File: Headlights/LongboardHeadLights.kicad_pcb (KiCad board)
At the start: 2 copper layers, 76.2 x 12.7 mm, 16 parts, among them P1 CONN_01X03, U1 AL8805

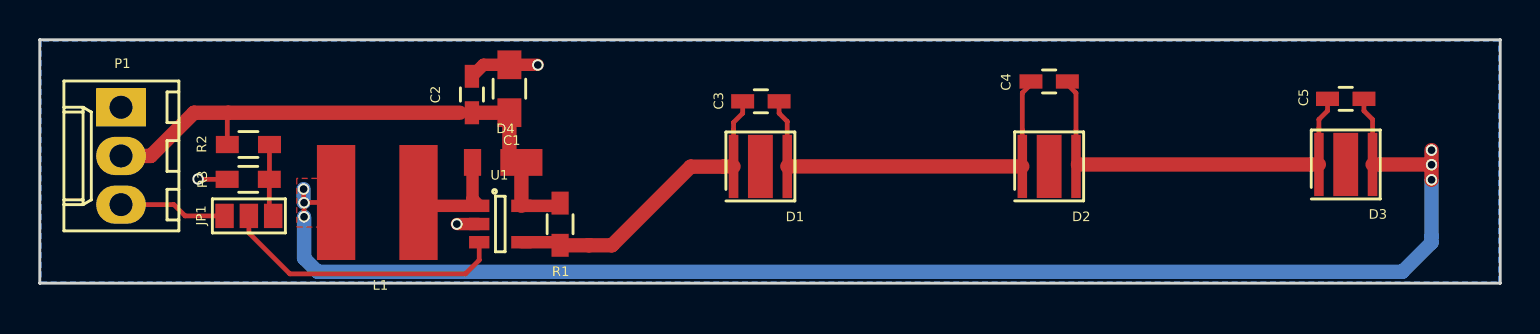
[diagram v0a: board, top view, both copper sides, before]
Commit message: updated project and completed rev 1 PCB
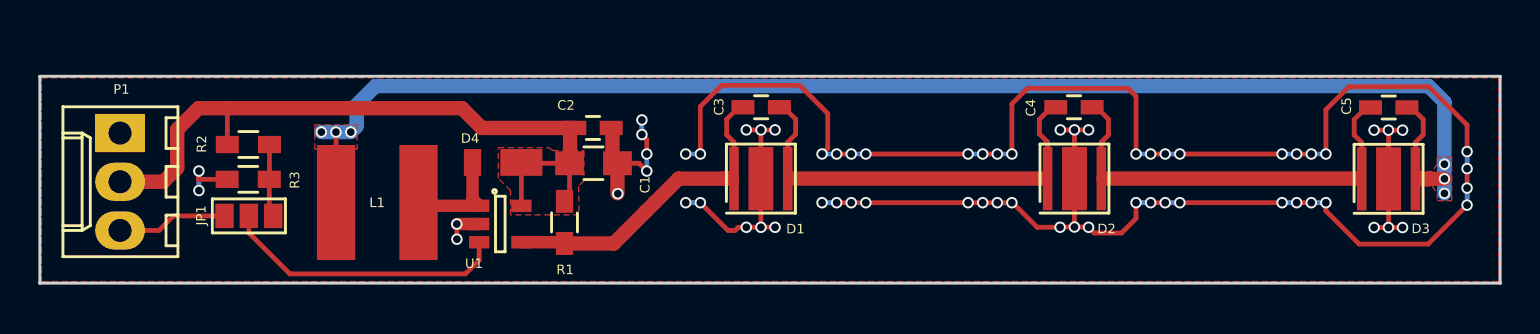
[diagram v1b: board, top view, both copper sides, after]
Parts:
- moved C2 6.55 mm to (155.1, 88.8), turned to 0 degrees
- moved C1 5.86 mm to (155.1, 90.7), turned to 0 degrees
- moved D3 2.36 mm to (196.6, 91.5)
- moved C5 2.29 mm to (196.6, 87.7)
- moved C4 1.87 mm to (180.1, 87.7)
- moved D2 1.47 mm to (180.2, 91.5)
- moved P1 1.35 mm to (130.4, 89.1)
- moved D1 0.64 mm to (163.8, 91.5)
- moved C3 0.31 mm to (163.8, 87.7)
- moved R1 0.25 mm to (153.6, 93.7)
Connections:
- D1 pad 3: (no net) -> GND
- D2 pad 3: (no net) -> GND
- D3 pad 3: (no net) -> GND
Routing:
- net GND: track 6.38 -> 137.1 mm, vias 3 -> 67
- net VCC: track 30.1 -> 37.8 mm
- net Net-(C5-Pad2): track 77.3 -> 74.7 mm
- net Net-(C3-Pad2): track 20.5 -> 22.0 mm
- net Net-(C4-Pad2): track 20.9 -> 22.2 mm
- net Net-(C3-Pad1): track 16.4 -> 17.0 mm
- added copper zone on F.Cu, net GND
- added copper zone on F.Cu, net VCC
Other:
- board size 76.2 x 12.7 mm -> 76.2 x 10.8 mm
